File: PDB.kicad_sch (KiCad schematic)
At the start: 32 parts, among them U13 B6B-XH-A(LF)(SN), U13 INA240A1QDRQ1, U14 TPS62933DRLR, U15 53.6k

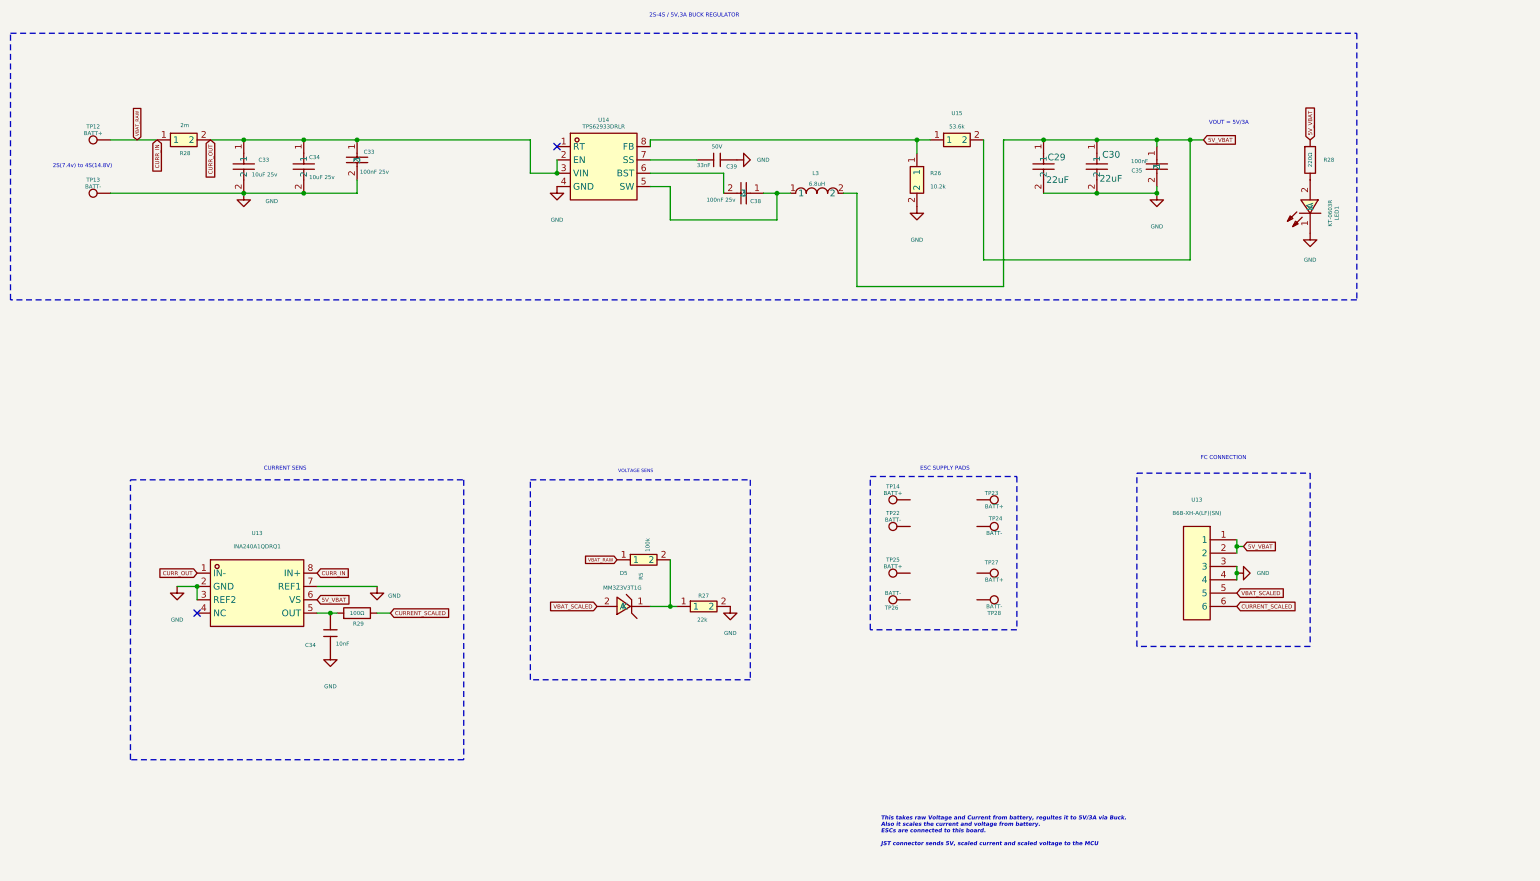
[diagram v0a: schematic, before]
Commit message: GPS connections made
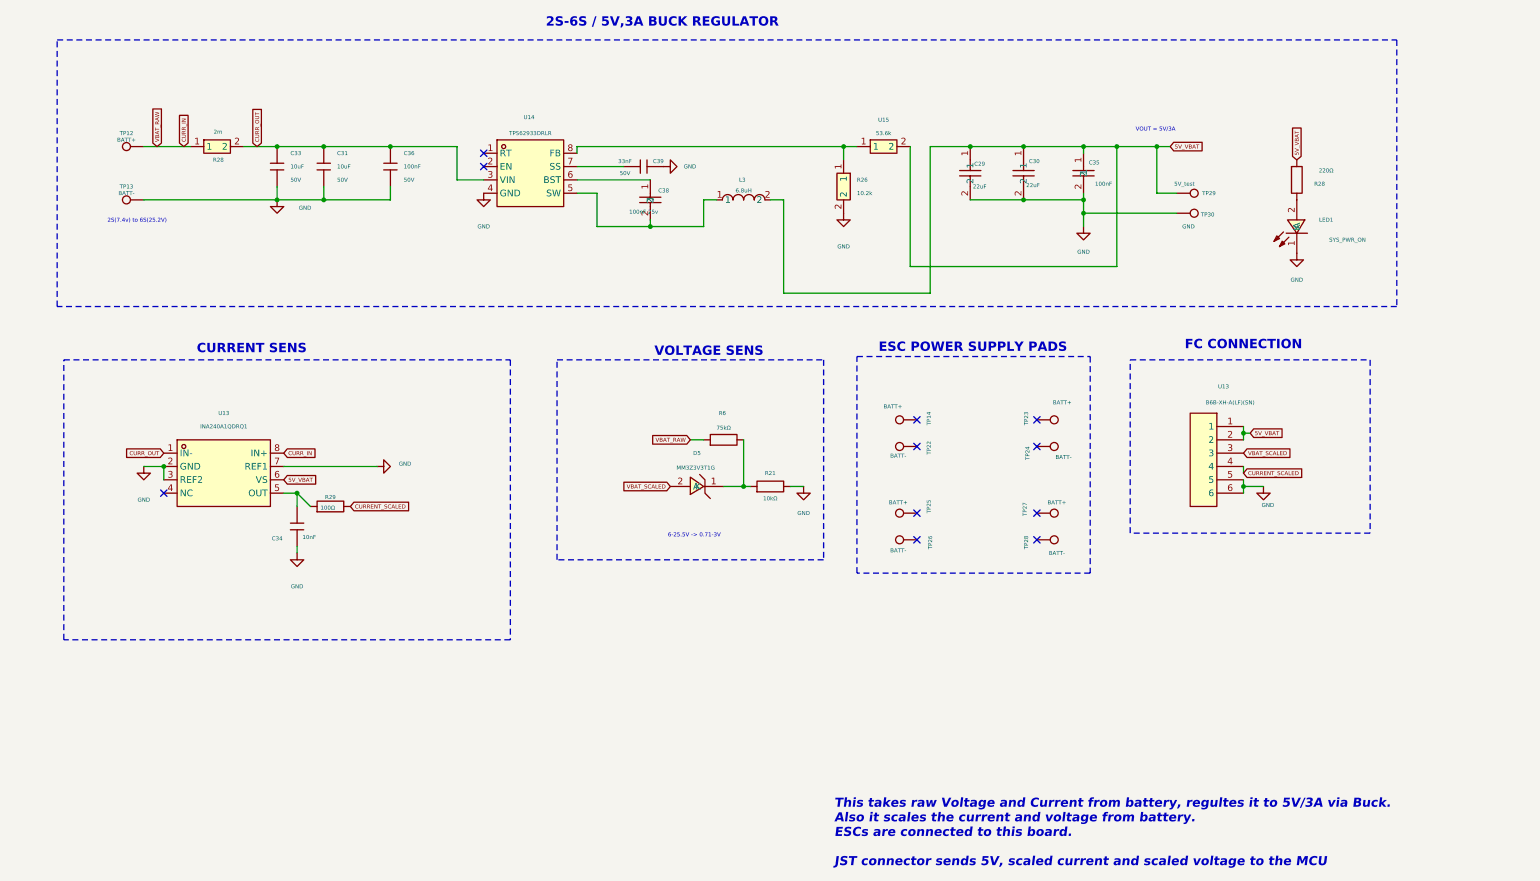
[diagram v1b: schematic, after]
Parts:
- removed C33: 100nF 25v, easyeda2kicad:C0402, symbol easyeda2kicad:CL05A104KA5NNNC
- removed C33, C34: 10uF 25v, easyeda2kicad:C0603, symbol easyeda2kicad:ZRB18AR61E106ME01L
- removed R27: 22k, easyeda2kicad:R0603, symbol easyeda2kicad:RT0603BRD0722KL
- removed R5: 100k, easyeda2kicad:R0603, symbol easyeda2kicad:RT0603BRD07100KL
- added C31, C33: 10uF, PCM_JLCPCB:C_0805, symbol PCM_JLCPCB-Capacitors:0805,10uF,(2)
- added C36: 100nF, PCM_JLCPCB:C_0402, symbol PCM_JLCPCB-Capacitors:0402,100nF,(2)
- added R21: 10kΩ, PCM_JLCPCB:R_0402, symbol PCM_JLCPCB-Resistors:0402,10kΩ
- added R6: 75kΩ, PCM_JLCPCB:R_0402, symbol PCM_JLCPCB-Resistors:0402,75kΩ
- added TP29: 5V_test, symbol Connector:TestPoint
- added TP30: GND, symbol Connector:TestPoint
- LED1: value KT-0603R -> SYS_PWR_ON
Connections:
- net 5V_VBAT: now also TP29.1
- net CURRENT_SCALED: now also U13.4; no longer U13.6
- net CURR_IN: now also R6.1
- net CURR_OUT: now also C31.1, C33.1, C36.1; no longer U14.2 (EN)
- net GND: now also U13.5, U13.6, C31.2, C33.2, C36.2, R21.2, TP30.1; no longer U13.3, U13.4
- net VBAT_SCALED: now also U13.3; no longer U13.5
- net at L3.1, U14.5 (SW): now also C38.2; no longer C38.1
- net at D5.1 (K): now also R21.1, R6.2
- net at U14.6 (BST): now also C38.1; no longer C38.2
- no-connect marks 2 -> 11
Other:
- note added: "2S(7.4v) to 6S(25.2V)"
- note added: "2S-6S / 5V,3A BUCK REGULATOR"
- note added: "6-25.5V -> 0.71-3V"
- note added: "ESC POWER SUPPLY PADS"
- note removed: "2S(7.4v) to 4S(14.8V)"
- note removed: "2S-4S / 5V,3A BUCK REGULATOR"
- note removed: "ESC SUPPLY PADS"
- moved on the sheet: C29, C30, C34, C35, C38, C39, D5, L3, LED1, R26, R28, R29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
